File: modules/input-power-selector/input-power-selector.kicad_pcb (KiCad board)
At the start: 2 copper layers, 61 x 47 mm, 37 parts, among them Q1 SI4909DY-T1-GE3, Q2 SI4909DY-T1-GE3, Q3 SI4909DY-T1-GE3, Q4 IPF067N20NM6ATMA1, Q7 BC847, U1 LTC4417IGN, U2 SQJQ141EL-T1_GE3

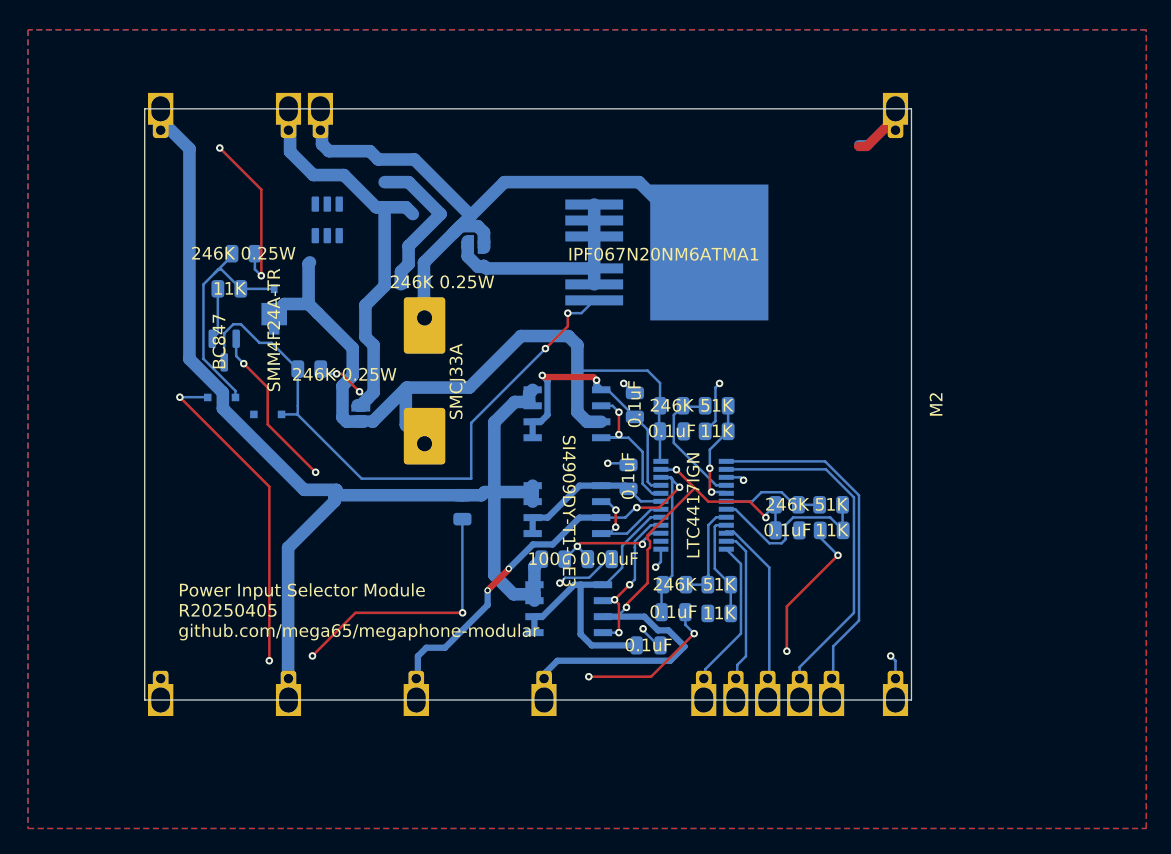
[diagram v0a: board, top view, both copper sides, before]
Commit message: Updating all modules
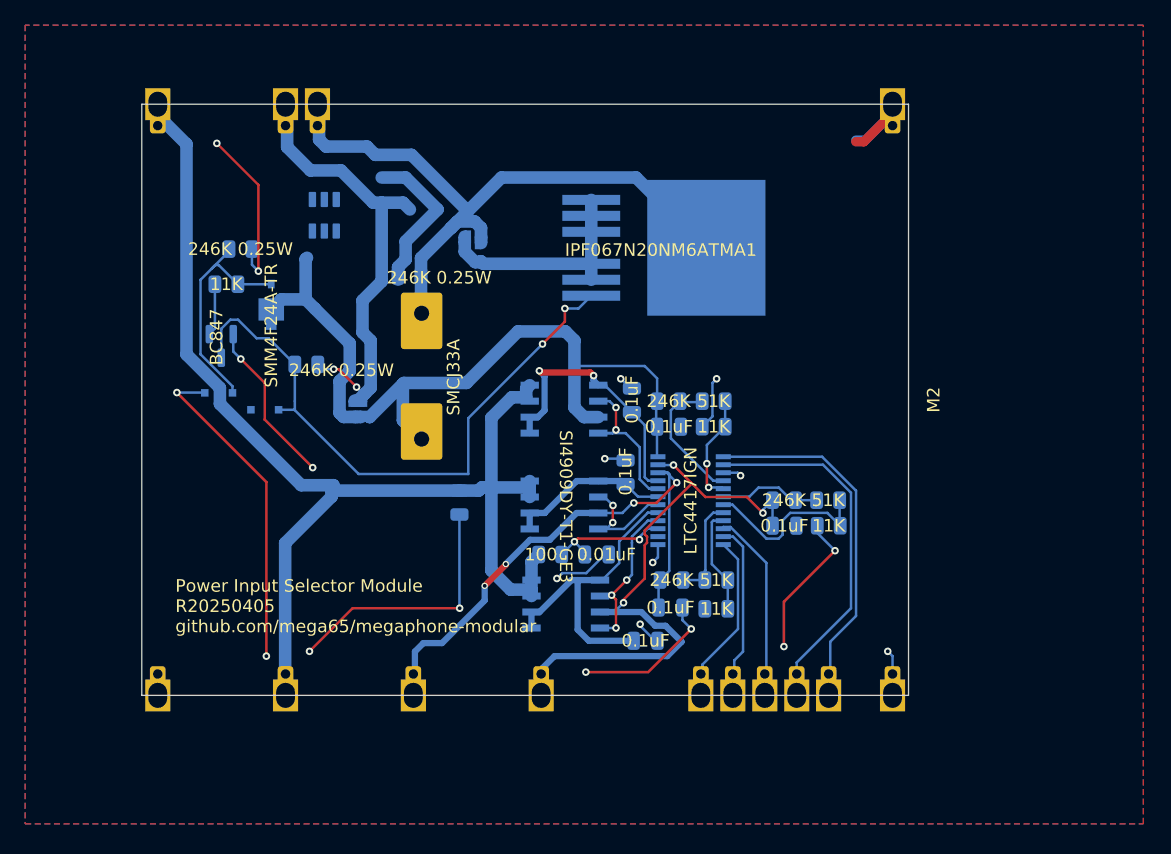
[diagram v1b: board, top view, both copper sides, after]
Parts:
- moved C7 0.44 mm to (63.8, 58.6)
- moved C8 0.44 mm to (72.8, 52.1)
- moved C9 0.44 mm to (57.9, 54.4)
- moved M2 0.44 mm to (52.2, 42.1)
- moved R10 0.44 mm to (54.2, 54.4)
- moved R12 0.44 mm to (34.8, 39.3)
- moved R14 0.44 mm to (43.0, 32.3)
- moved R2 0.44 mm to (67.2, 42.2)
- moved R7 0.44 mm to (76.4, 52.1)
- moved U1 0.44 mm to (65.4, 50.1)
- moved D2 0.44 mm to (31.5, 42.9)
- moved Q7 0.44 mm to (28.1, 37.8)
- moved R13 0.44 mm to (28.5, 32.9)
- moved D3 0.44 mm to (44.2, 27.0)
- moved U2 0.44 mm to (36.3, 27.4)
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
